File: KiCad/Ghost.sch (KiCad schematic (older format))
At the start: 16 parts, among them P1 CONN_01X02, Q1 MMBT3904 (SOT-23), U1 INA219, U2 Teensy31_32, U3 MIC5219-3.3YM5

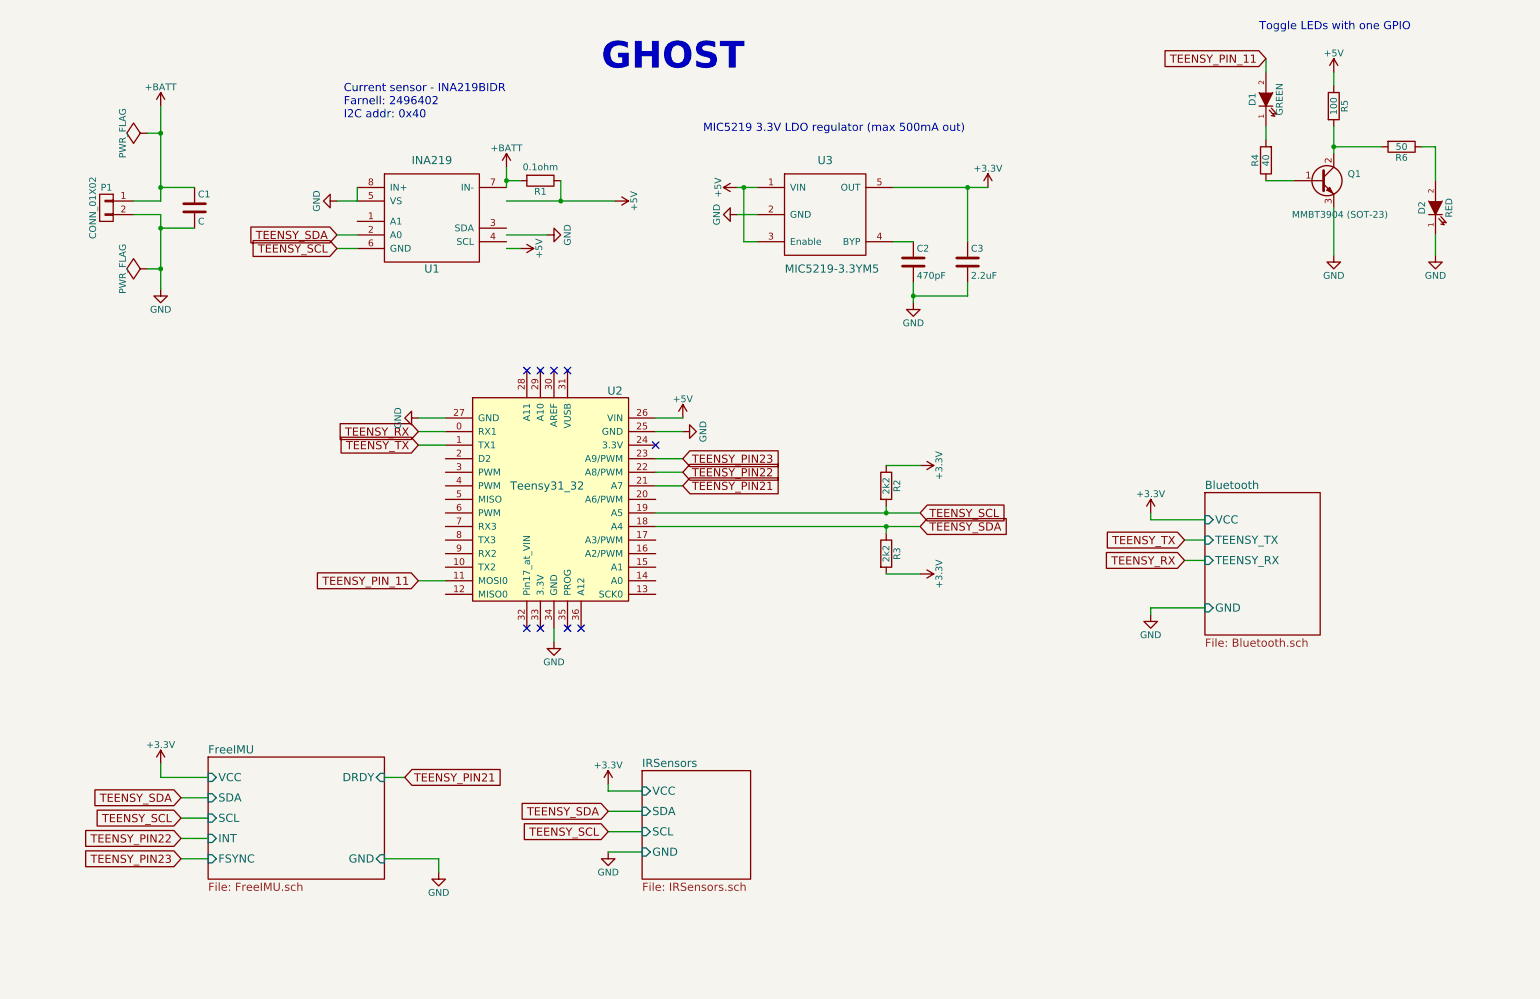
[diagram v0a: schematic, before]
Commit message: Lots of changes
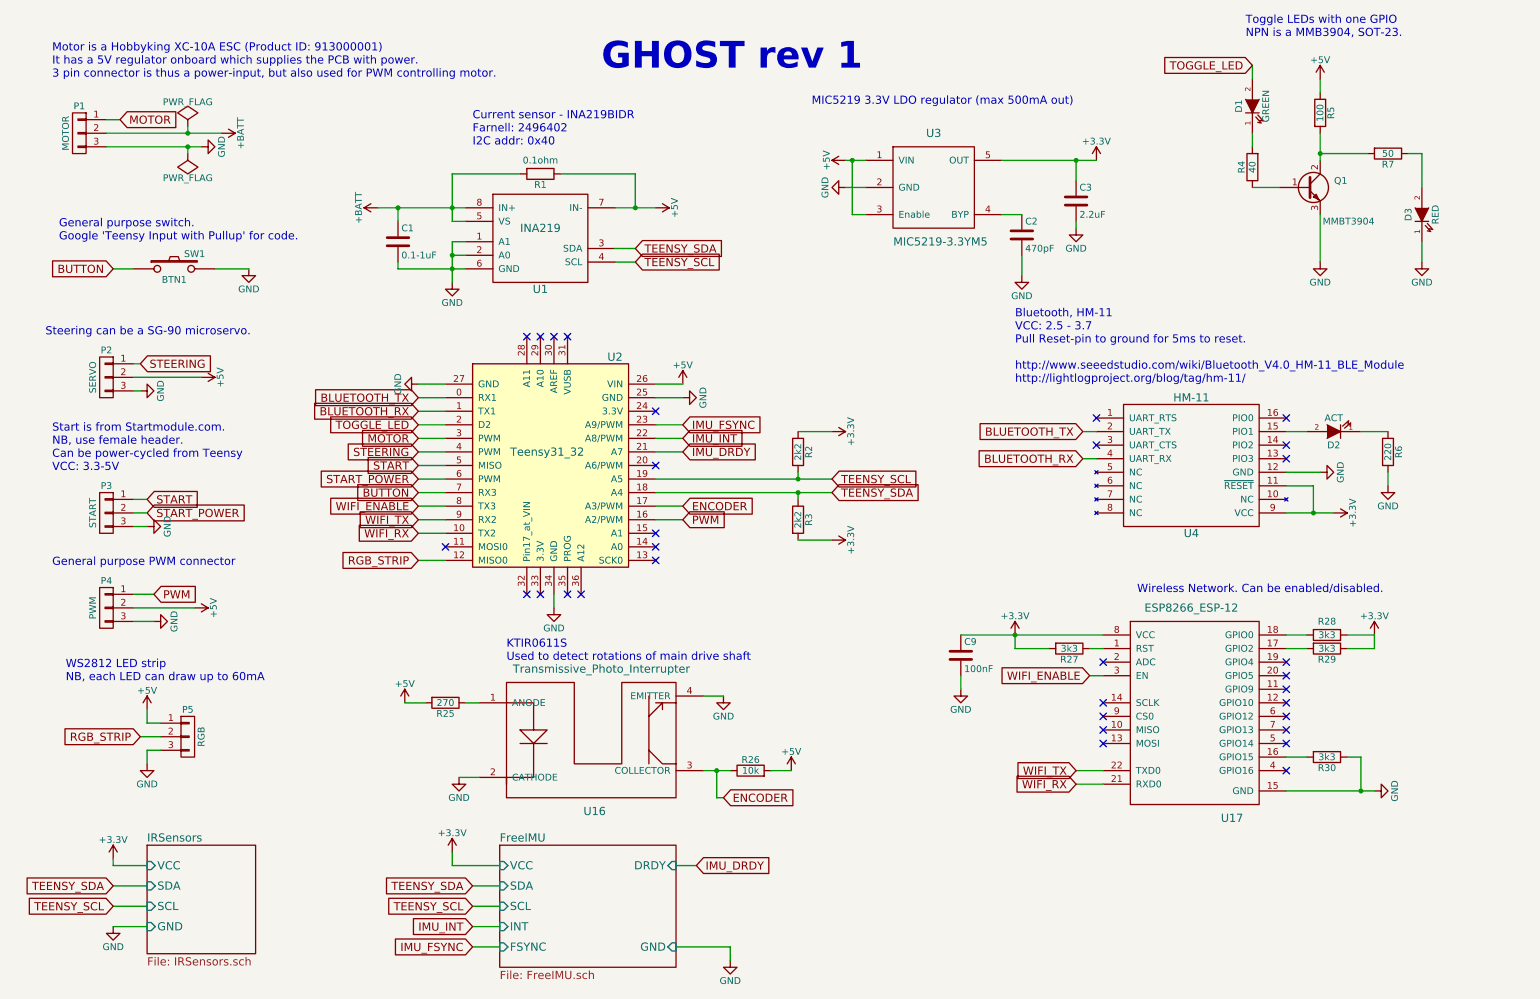
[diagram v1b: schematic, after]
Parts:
- removed P1: CONN_01X02, symbol CONN_01X02
- added C9: 100nF, Capacitors_SMD:C_0805, symbol C
- added D2: ACT, LEDs:LED_0805, symbol LED
- added P1: MOTOR, Pin_Headers:Pin_Header_Straight_1x03, symbol CONN_01X03
- added P2: SERVO, Pin_Headers:Pin_Header_Straight_1x03, symbol CONN_01X03
- added P3: START, Pin_Headers:Pin_Header_Straight_1x03, symbol CONN_01X03
- added P4: PWM, Pin_Headers:Pin_Header_Straight_1x03, symbol CONN_01X03
- added P5: RGB, Pin_Headers:Pin_Header_Straight_1x03, symbol CONN_01X03
- added R25: 270, Resistors_SMD:R_0805, symbol R
- added R26: 10k, Resistors_SMD:R_0805, symbol R
- added R27, R28, R29, R30: 3k3, Resistors_SMD:R_0805, symbol R
- added R6: 220, Resistors_SMD:R_0805, symbol R
- added SW1: BTN1, Buttons_Switches_SMD:SW_SPST_SKQG, symbol SW_PUSH
- added U16: Transmissive_Photo_Interrupter, Pin_Headers:Pin_Header_Straight_1x04, symbol Transmissive_Photo_Interrupter
- added U17: ESP8266_ESP-12, NorBotKiCadFootprints:ESP8266_ESP_12E, symbol ESP8266_ESP-12
- added U4: HM-11, NorBotKiCadFootprints:HM-11, symbol HM-11
- C1: value C -> 0.1-1uF
- Q1: value MMBT3904 (SOT-23) -> MMBT3904
- U2: footprint (none) -> NorBotKiCadFootprints:Teensy-3.1_3.2
- renumbered D2 to D3, R6 to R7
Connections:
- net labels added: BLUETOOTH_RX, BLUETOOTH_TX, BUTTON, ENCODER, IMU_DRDY, IMU_FSYNC, IMU_INT, MOTOR, PWM, RGB_STRIP, START, START_POWER, STEERING, TOGGLE_LED, WIFI_ENABLE, WIFI_RX, WIFI_TX
- net labels removed: TEENSY_PIN21, TEENSY_PIN22, TEENSY_PIN23, TEENSY_PIN_11, TEENSY_RX, TEENSY_TX
- wire segments 74 -> 130
- no-connect marks 9 -> 32
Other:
- note added: "Bluetooth, HM-11\nVCC: 2.5 - 3.7\nPull Reset-pin to ground for 5ms to reset.\n\nhttp://www.seeedstudio.com/wiki/Bluetooth_V4.0_HM-11_BLE_Module\nhttp://lightlogproject.org/blog/tag/hm-11/"
- note added: "GHOST rev 1"
- note added: "General purpose PWM connector"
- note added: "General purpose switch.\nGoogle 'Teensy Input with Pullup' for code."
- note added: "KTIR0611S\nUsed to detect rotations of main drive shaft"
- note added: "Motor is a Hobbyking XC-10A ESC (Product ID: 913000001)\nIt has a 5V regulator onboard which supplies the PCB with power.\n3 pin connector is thus a power-input, but also used for PWM controlling motor."
- note added: "Start is from Startmodule.com.\nNB, use female header.\nCan be power-cycled from Teensy\nVCC: 3.3-5V"
- note added: "Steering can be a SG-90 microservo."
- note added: "Toggle LEDs with one GPIO\nNPN is a MMB3904, SOT-23."
- note added: "WS2812 LED strip\nNB, each LED can draw up to 60mA"
- note added: "Wireless Network. Can be enabled/disabled."
- note removed: "GHOST"
- note removed: "Toggle LEDs with one GPIO"
- moved on the sheet: C1, C2, C3, D1, D3, Q1, R1, R2, R3, R4, R5, R7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
